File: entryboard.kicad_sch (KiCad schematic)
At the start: 25 parts, among them J1 Conn_01x01, J10 Conn_01x01, J11 Conn_01x01, J12 Conn_01x01, J13 Conn_01x03_Pin, J14 USB_C_Receptacle, J15 Conn_01x03_Pin, J16 Conn_01x01_Pin, J2 Conn_01x01, J3 Conn_01x01, J4 Conn_01x01, J5 Conn_01x01, J6 Conn_01x01, J7 Conn_01x01, J8 USB_A, J9 Conn_01x02_Pin, SW1 SW_Push, SW2 SW_Push, SW3 SW_Push

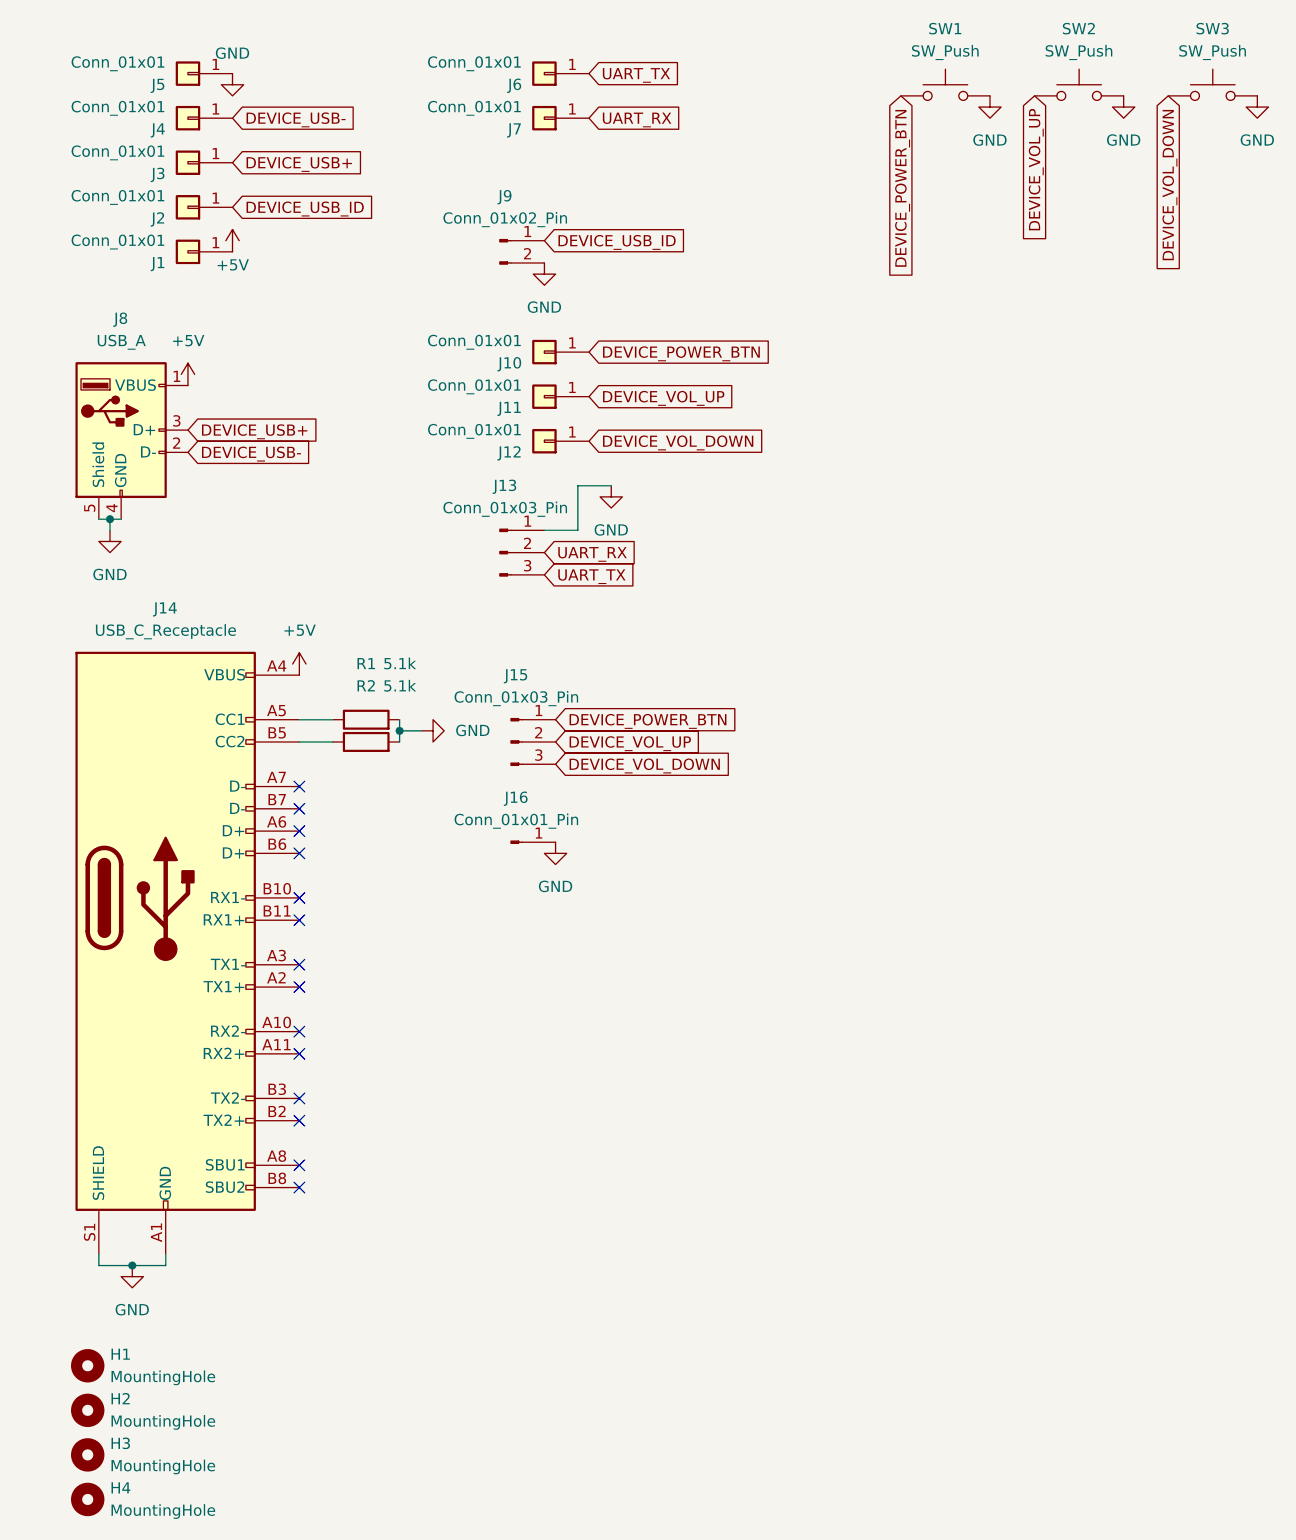
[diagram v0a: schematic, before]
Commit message: too much to say
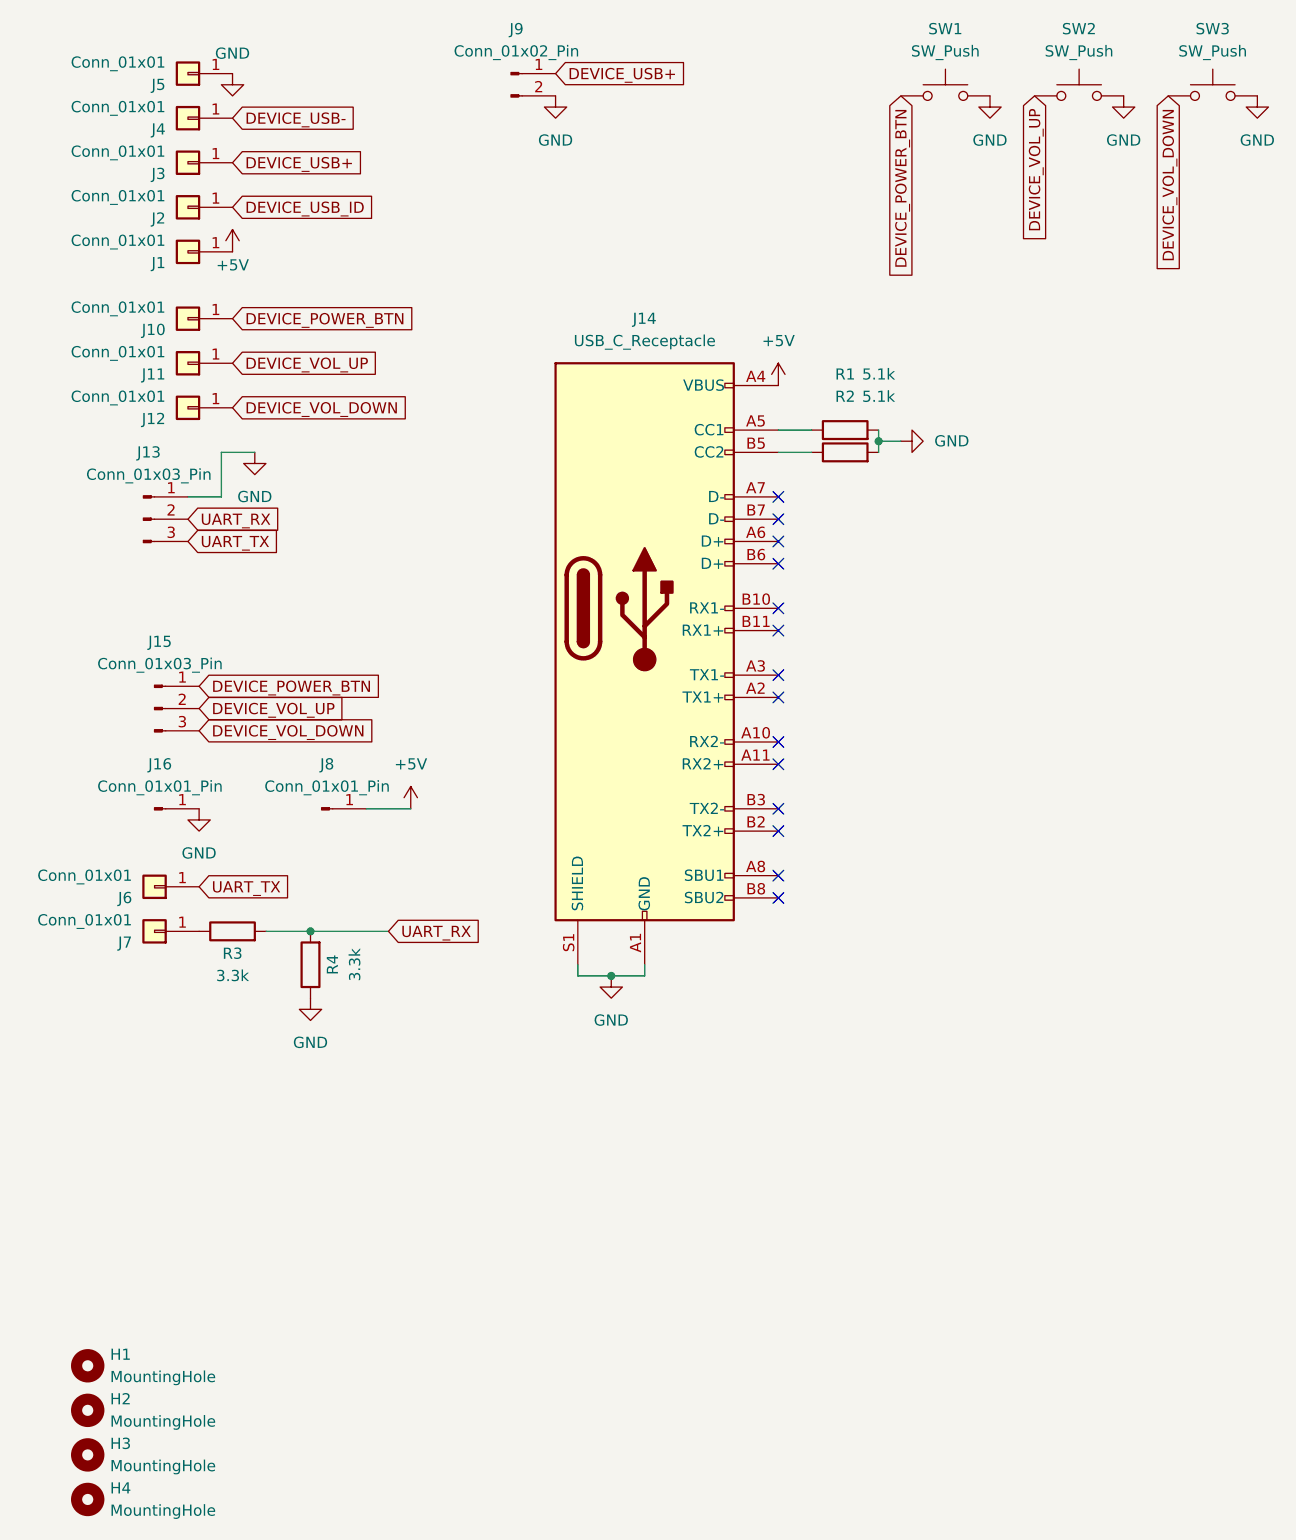
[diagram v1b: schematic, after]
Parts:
- removed J8: USB_A, Connector_USB:USB_A_Kycon_KUSBX-AS1N-B_Horizontal, symbol Connector:USB_A
- added J8: Conn_01x01_Pin, Connector_PinHeader_1.00mm:PinHeader_1x01_P2.54mm_Vertical, symbol Connector:Conn_01x01_Pin
- added R3, R4: 3.3k, Resistor_SMD:R_1206_3216Metric_Pad1.30x1.75mm_HandSolder, symbol Device:R
- J1, J10, J11, J12, J2, J3, J4, J5: footprint TestPoint:TestPoint_Pad_1.0x1.0mm -> Connector_PinSocket_2.54mm:PinSocket_1x01_P2.54mm_Vertical
- J16: footprint Connector_PinHeader_1.00mm:PinHeader_1x01_P1.00mm_Vertical -> Connector_PinHeader_2.54mm:PinHeader_1x01_P2.54mm_Vertical
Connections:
- net +5V: now also J8.1 (Pin_1)
- net DEVICE_USB+: now also J9.1 (Pin_1)
- net DEVICE_USB_ID: no longer J9.1 (Pin_1)
- net GND: now also R4.1
- net UART_RX: now also R3.2, R4.2; no longer J7.1 (Pin_1)
- new net: J7.1 (Pin_1), R3.1
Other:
- moved on the sheet: J11, J13, J14, J15, J16, J6, J7, J9, R1, R2
